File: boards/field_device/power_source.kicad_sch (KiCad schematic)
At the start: 9 parts, among them U4 CN3163

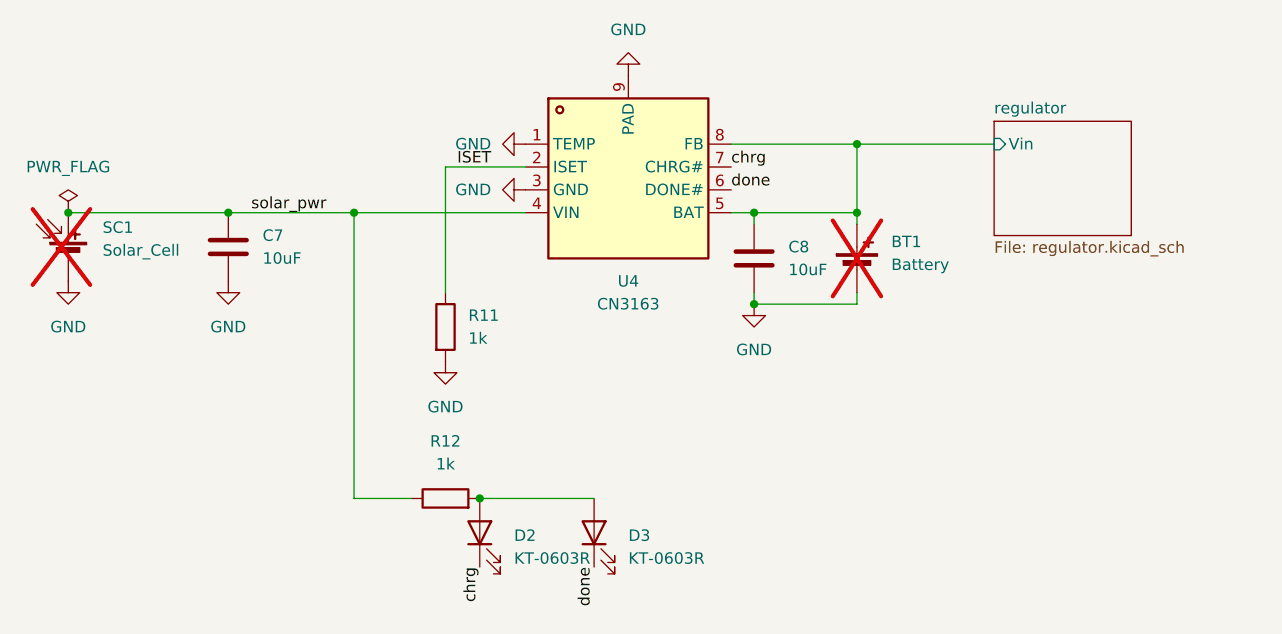
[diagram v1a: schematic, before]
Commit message: idk atp
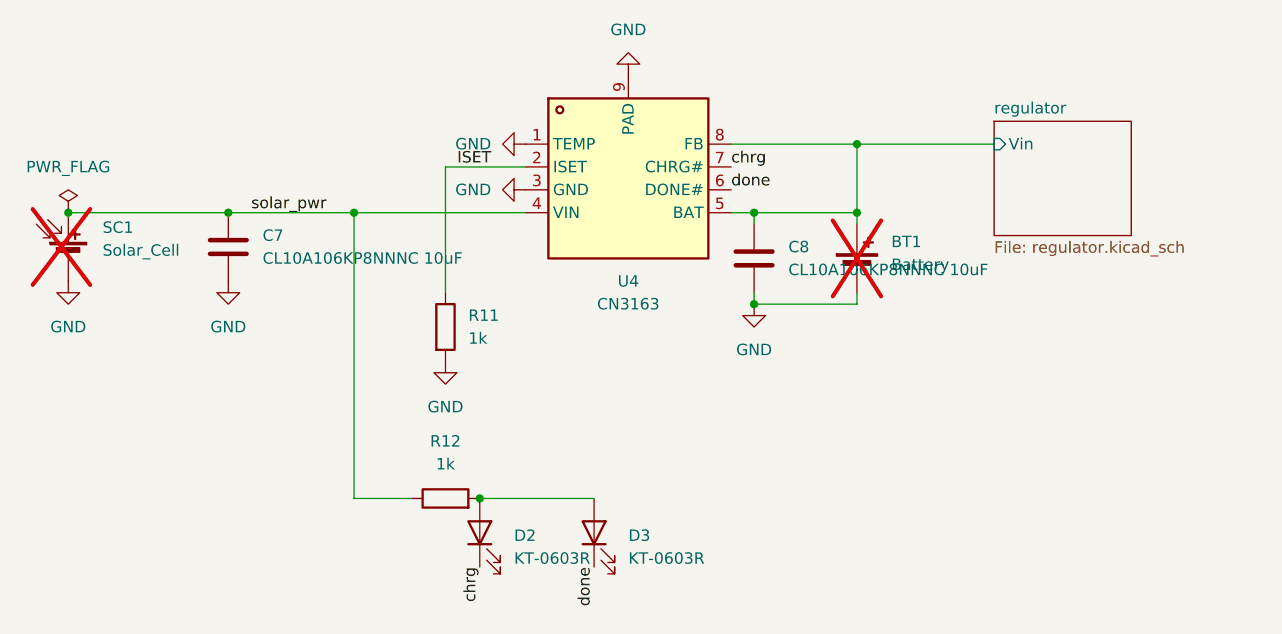
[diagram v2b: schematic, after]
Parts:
- C7, C8: value 10uF -> CL10A106KP8NNNC 10uF
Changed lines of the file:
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@@
 			)
 		)
-		(property "Value" "10uF"
+		(property "Value" "CL10A106KP8NNNC 10uF"
 			(at 110.49 52.0699 0)
 			(show_name no)
@@
 			)
 		)
-		(property "Value" "10uF"
+		(property "Value" "CL10A106KP8NNNC 10uF"
 			(at 52.07 50.7999 0)
 			(show_name no)
